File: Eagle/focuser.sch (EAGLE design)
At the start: 46 parts, among them IC1 78xx, J1 J5MM, J10 J5MM, J2 J7MM, J3 J7MM, J4 J5MM, J5 J7MM, J6 J12MM, J7 J7MM, J8 J7MM, J9 J5MM, U1 L298

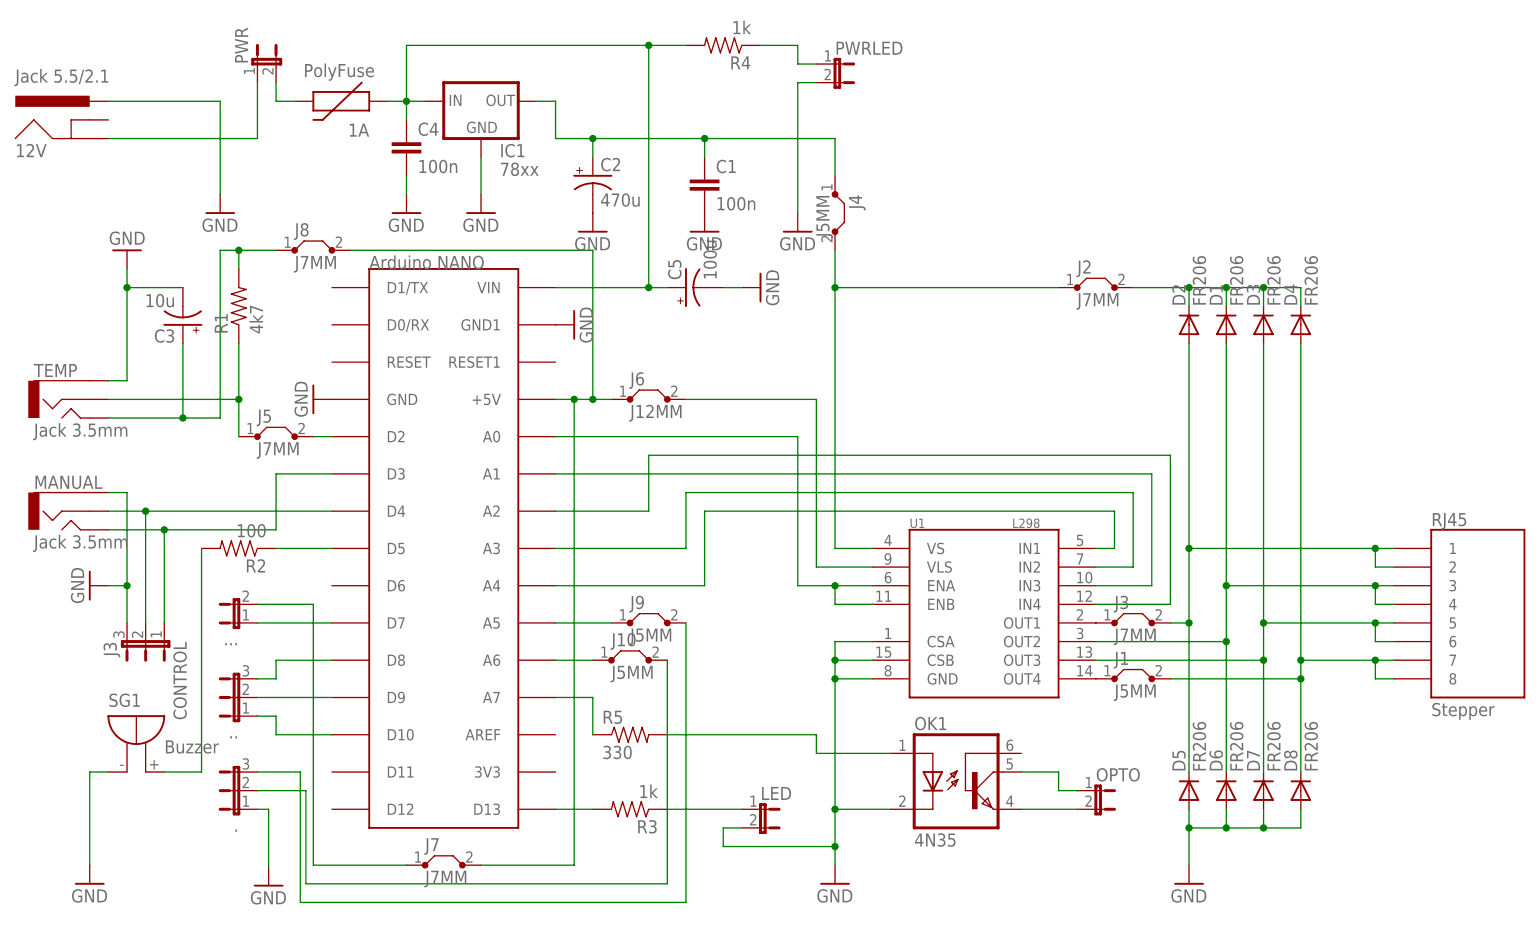
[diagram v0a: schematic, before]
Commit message: Focuser 2.0
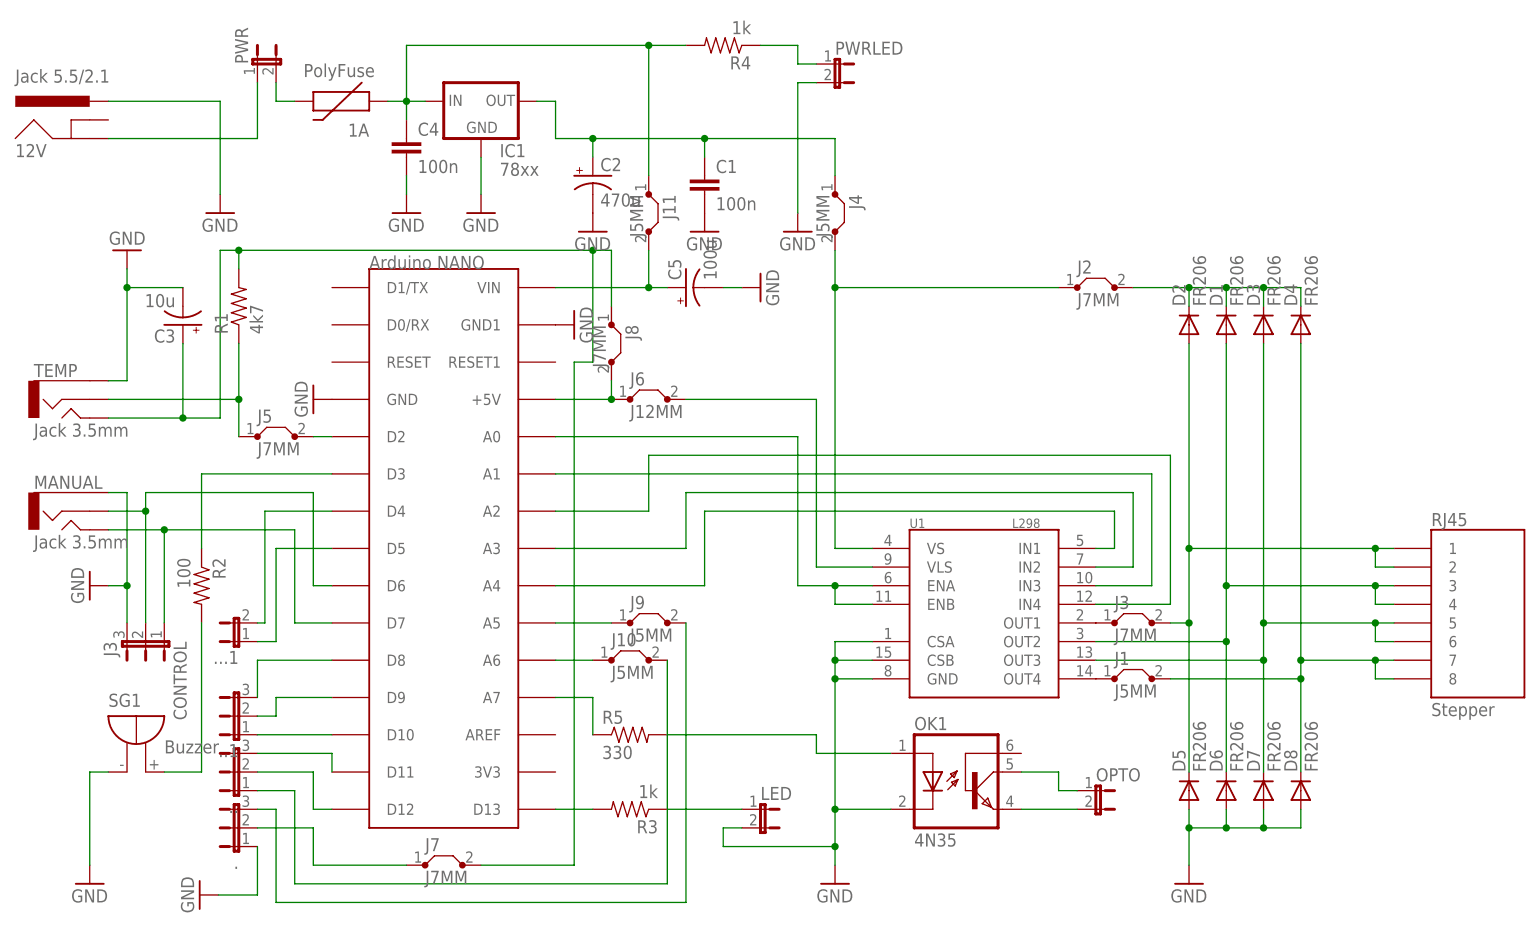
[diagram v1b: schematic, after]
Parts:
- removed ...: (no value), SparkFun:JUMPER-2PTH
- added ...1: (no value), SparkFun:JUMPER-2PTH
- added ..1: JUMPER-3PTH, SparkFun:JUMPER-3PTH
- added J11: J5MM, jumper:J5MM
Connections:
- removed net N$30: C3.+, J8.1, R1.2, TEMP.5
- new net N$41: ..1.1, NANO.D10
- new net N$42: ...3, NANO.D11
- new net N$43: ...2, NANO.D12
- new net N$44: C5.+, J11.2, NANO.VIN
- new net N$45: J6.1, J8.2, NANO.+5V
- net +5: now also C3.+, J8.1, R1.2, TEMP.5; no longer J6.1, J8.2, NANO.+5V
- net N$18: now also NANO.D6; no longer NANO.D4
- net N$24: now also NANO.D7; no longer NANO.D3
- net N$31: now also ...1; no longer ..2
- net N$32: now also ...1.2, NANO.D4; no longer ...3, NANO.D8
- net N$33: now also ...1.1, NANO.D5; no longer ...2, NANO.D9
- net N$34: now also ..1.3, NANO.D8; no longer ...1, NANO.D10
- net N$35: now also ..1.2, NANO.D9; no longer NANO.D5, R2.1
- net N$6: now also ..2; no longer ....2
- net N$8: now also NANO.D3, R2.1; no longer ....1, NANO.D7
- net N$9: now also J11.1; no longer C5.+, NANO.VIN
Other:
- moved on the sheet: ., .., J8, R2
